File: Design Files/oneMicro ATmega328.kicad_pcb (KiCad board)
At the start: 2 copper layers, 18 x 35.3 mm, 28 parts, among them CON1 USB-MINI-B, IC1 ATMEGA328-P, IC2 MIC5205, P14 CONN_01X01, P2 CONN_01X12, P3 CONN_01X02, P5 CONN_01X12, SW1 RESET, U1 CP2102, X1 16MHz

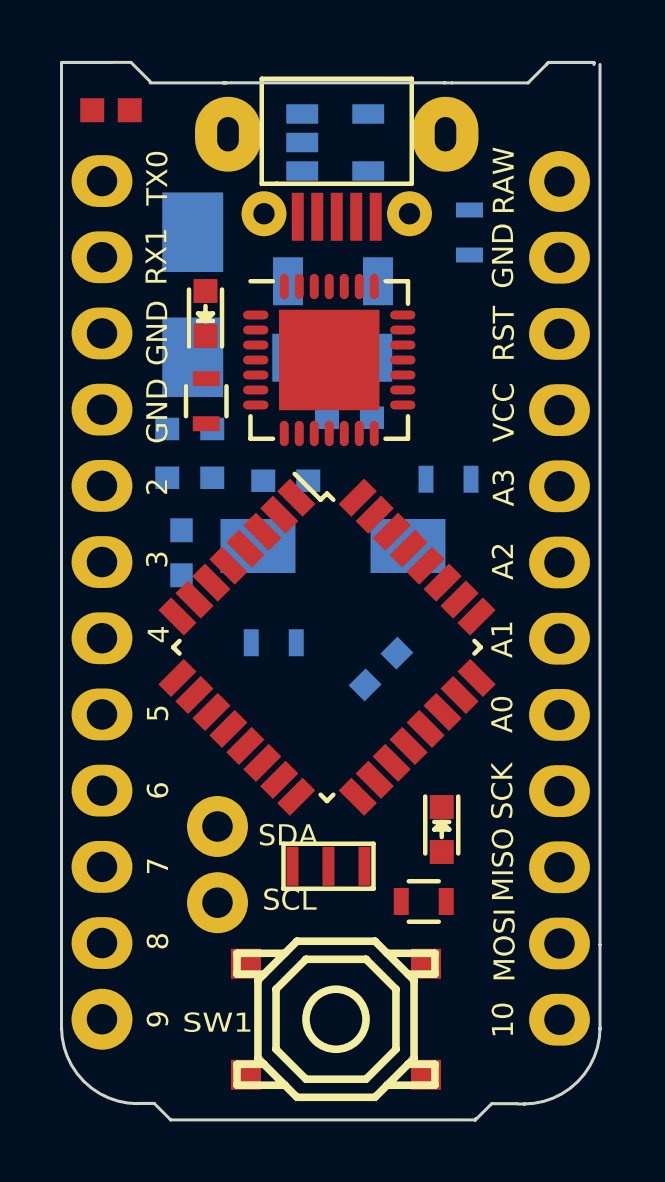
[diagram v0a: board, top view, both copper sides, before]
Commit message: Design Completed
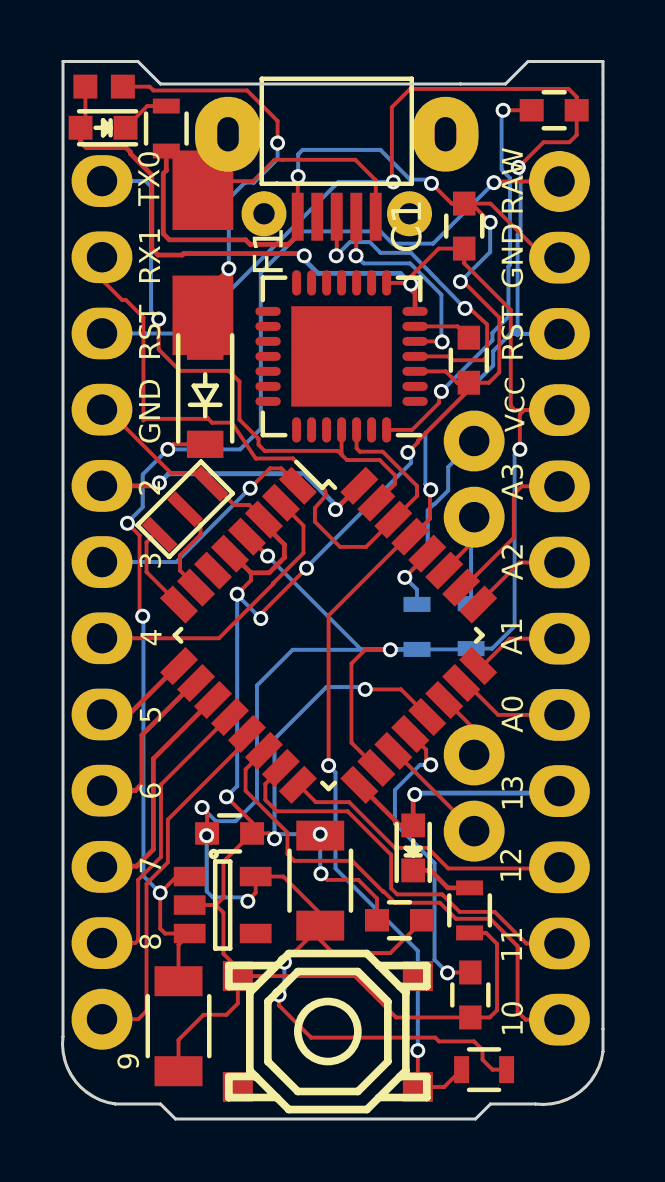
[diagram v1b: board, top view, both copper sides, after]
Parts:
- added P1: CONN_01X02, Pin_Headers:Pin_Header_Straight_1x02, F.Cu at (165.5, 116.2)
- C1, C2, C3, C4, C6, C7, C8, C9, F1, IC2, R3: moved to F.Cu
- D4: footprint EE:ZenerDiode_SMD_new -> Diodes_SMD:SOD-123; moved to F.Cu
- IC1: value ATMEGA328-P -> ATMEGA328P-A
- moved IC2 25.7 mm to (157.1, 118.6)
- moved C7 25.4 mm to (155.6, 122.7), turned to 270 degrees
- moved C3 17.8 mm to (163.0, 119.1)
- moved C8 17.4 mm to (160.3, 117.8), turned to 90 degrees
- moved R3 15.9 mm to (165.8, 124.1), turned to 180 degrees
- moved C6 15.2 mm to (168.1, 92.1), turned to 180 degrees
- moved C9 14.4 mm to (157.3, 116.2)
- moved C1 14.4 mm to (165.1, 96.0)
- moved P3 13.4 mm to (165.5, 105.7), turned to 180 degrees
- moved R2 13.1 mm to (165.4, 109.3), turned to 270 degrees
- moved C2 11.3 mm to (165.3, 121.6), turned to 270 degrees
- moved X1 10.1 mm to (156.8, 106.5), turned to 45 degrees
- moved C4 10.1 mm to (165.3, 100.5), turned to 270 degrees
- moved R8 9.19 mm to (155.2, 92.7)
- moved D3 7.07 mm to (153.1, 92.7), turned to 180 degrees
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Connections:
- D1 pad 1: /SCK -> Net-(D1-Pad1)
- D1 pad 2: Net-(D1-Pad2) -> /SCK
- IC1 pad 1: /RESET -> /D3
- IC1 pad 10: Net-(IC1-Pad10) -> /D6
- IC1 pad 11: /D5 -> /D7
- IC1 pad 12: /D6 -> /D8
- IC1 pad 13: /D7 -> /D9
- IC1 pad 14: /D8 -> /D10
- IC1 pad 15: /D9 -> /MOSI
- IC1 pad 16: /D10 -> /MISO
- IC1 pad 17: /MOSI -> /SCK
- IC1 pad 18: /MISO -> VCC
- IC1 pad 19: /SCK -> /A6
- IC1 pad 2: /RXD -> /D4
- IC1 pad 20: VCC -> Net-(C2-Pad1)
- IC1 pad 21: Net-(C2-Pad1) -> GND
- IC1 pad 22: GND -> /A7
- IC1 pad 29: (no net) -> /RESET
- IC1 pad 3: /TXD -> GND
- IC1 pad 30: (no net) -> /RXD
- IC1 pad 31: (no net) -> /TXD
- IC1 pad 32: (no net) -> /D2
- IC1 pad 4: /D2 -> VCC
- IC1 pad 5: /D3 -> GND
- IC1 pad 6: /D4 -> Net-(IC1-Pad6)
- IC1 pad 7: VCC -> Net-(IC1-Pad7)
- IC1 pad 9: Net-(IC1-Pad9) -> /D5
- P2 pad 10: GND -> /RESET
- P2 pad 11: /RXD1 -> /RXD
- P2 pad 12: /TXD0 -> /TXD
- R4 pad 1: VCC -> GND
- R4 pad 2: Net-(D1-Pad2) -> Net-(D1-Pad1)
- X1 pad 1: Net-(IC1-Pad10) -> Net-(IC1-Pad8)
- X1 pad 2: Net-(IC1-Pad9) -> Net-(IC1-Pad7)
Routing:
- net GND: track 0.00 -> 103.1 mm, vias 0 -> 13
- net VCC: track 0.00 -> 90.5 mm, vias 0 -> 10
- net /RESET: track 0.00 -> 63.5 mm, vias 0 -> 5
- net /RAW: track 0.00 -> 42.4 mm, vias 0 -> 5
- net /RXD: track 0.00 -> 22.5 mm
- net /TXD: track 0.00 -> 19.7 mm, vias 0 -> 1
- net /D10: track 0.00 -> 16.9 mm
- net Net-(D4-Pad1): track 0.00 -> 14.4 mm, vias 0 -> 2
- net Net-(C6-Pad2): track 0.00 -> 13.9 mm, vias 0 -> 2
- net /MOSI: track 0.00 -> 13.7 mm
- net /D9: track 0.00 -> 12.3 mm
- net Net-(CON1-Pad3): track 0.00 -> 11.2 mm, vias 0 -> 2
- net Net-(C2-Pad1): track 0.00 -> 10.4 mm, vias 0 -> 2
- net /D8: track 0.00 -> 10.1 mm
- net /D4: track 0.00 -> 10.1 mm
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- added copper zone on B.Cu, net GND
- added copper zone on F.Cu, net VCC
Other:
- board size 18 x 35.3 mm -> 18 x 35.2 mm
- net class Default: clearance 0.1651 -> 0.1
- rule trace_clearance: 0.1651 -> 0.1
- rule trace_min: 0.254 -> 0.13
- rule via_min_size: 0.6 -> 0.5
- board text added: "11"
- board text added: "12"
- board text added: "13"
- board text added: "ATmega328"
- board text added: "ExploreEmbedded"
- board text added: "oneMicro"
- board text removed: "MISO"
- board text removed: "MOSI"
- board text removed: "SCK"
- board text removed: "SCL"
- board text removed: "SDA"
